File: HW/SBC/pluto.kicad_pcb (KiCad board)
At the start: 2 copper layers, 120.7 x 108 mm, 42 parts, among them J1 Serial Port, J2 CONN_02X07, J3 CONN_02X07, J4 POWER IN, J5 Expansion Port, Q1 DS1813, SW1 RESET, U1 WD65C02_, U10 74LS138, U11 LM7805CT, U2 28C256, U3 HM62256BLP-7, U4 MAX232, U5 6551, U6 WD65C22, U7 DS1511Y+, U8 74HCT00, U9 74LS30, X1 4 MHz

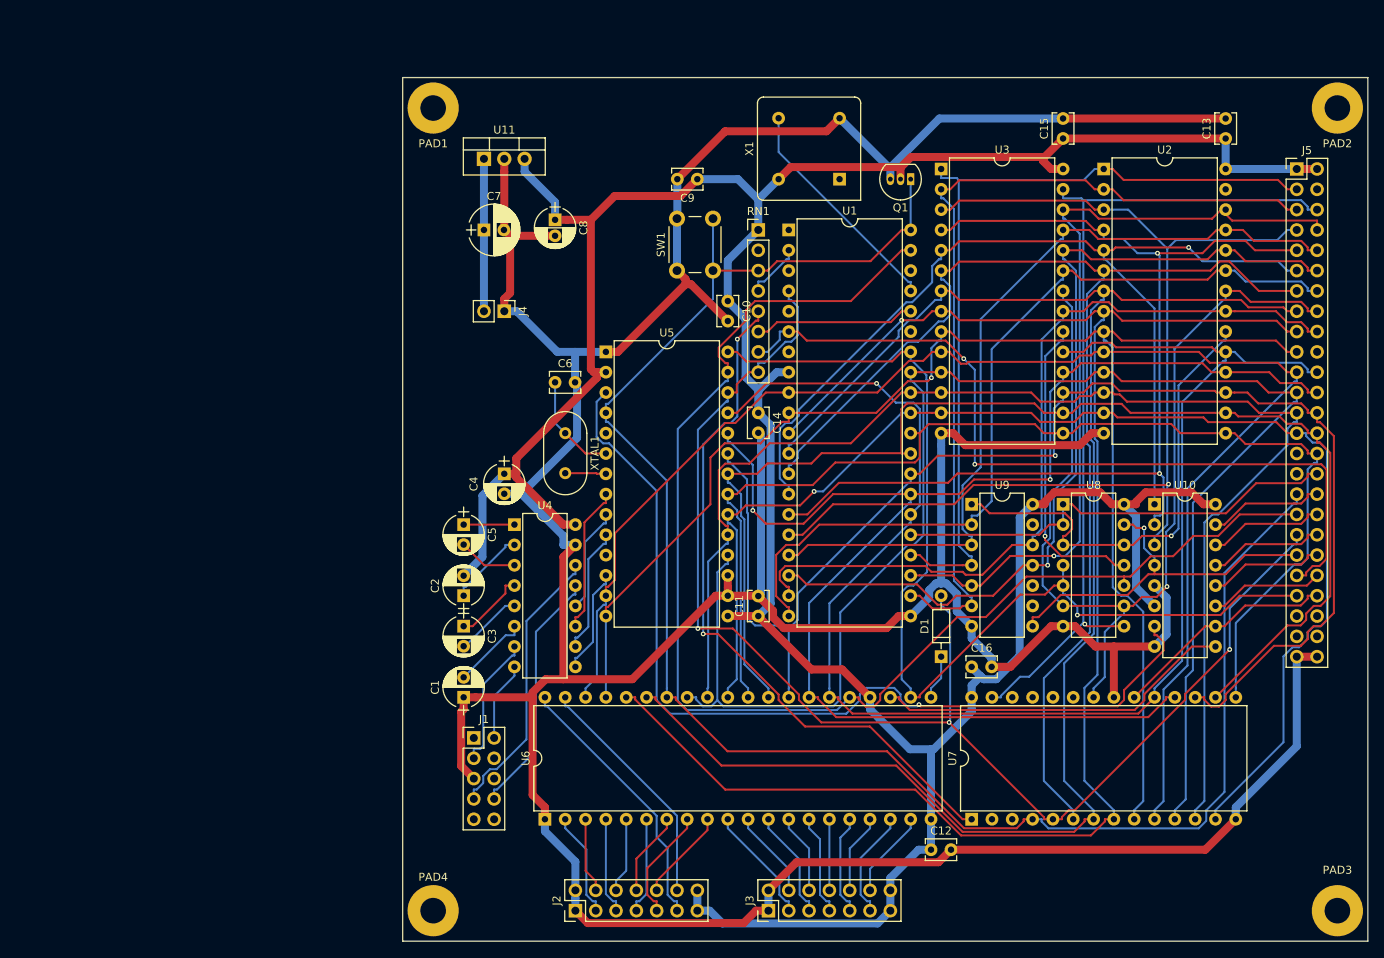
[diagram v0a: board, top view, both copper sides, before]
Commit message: New board layout. WIP
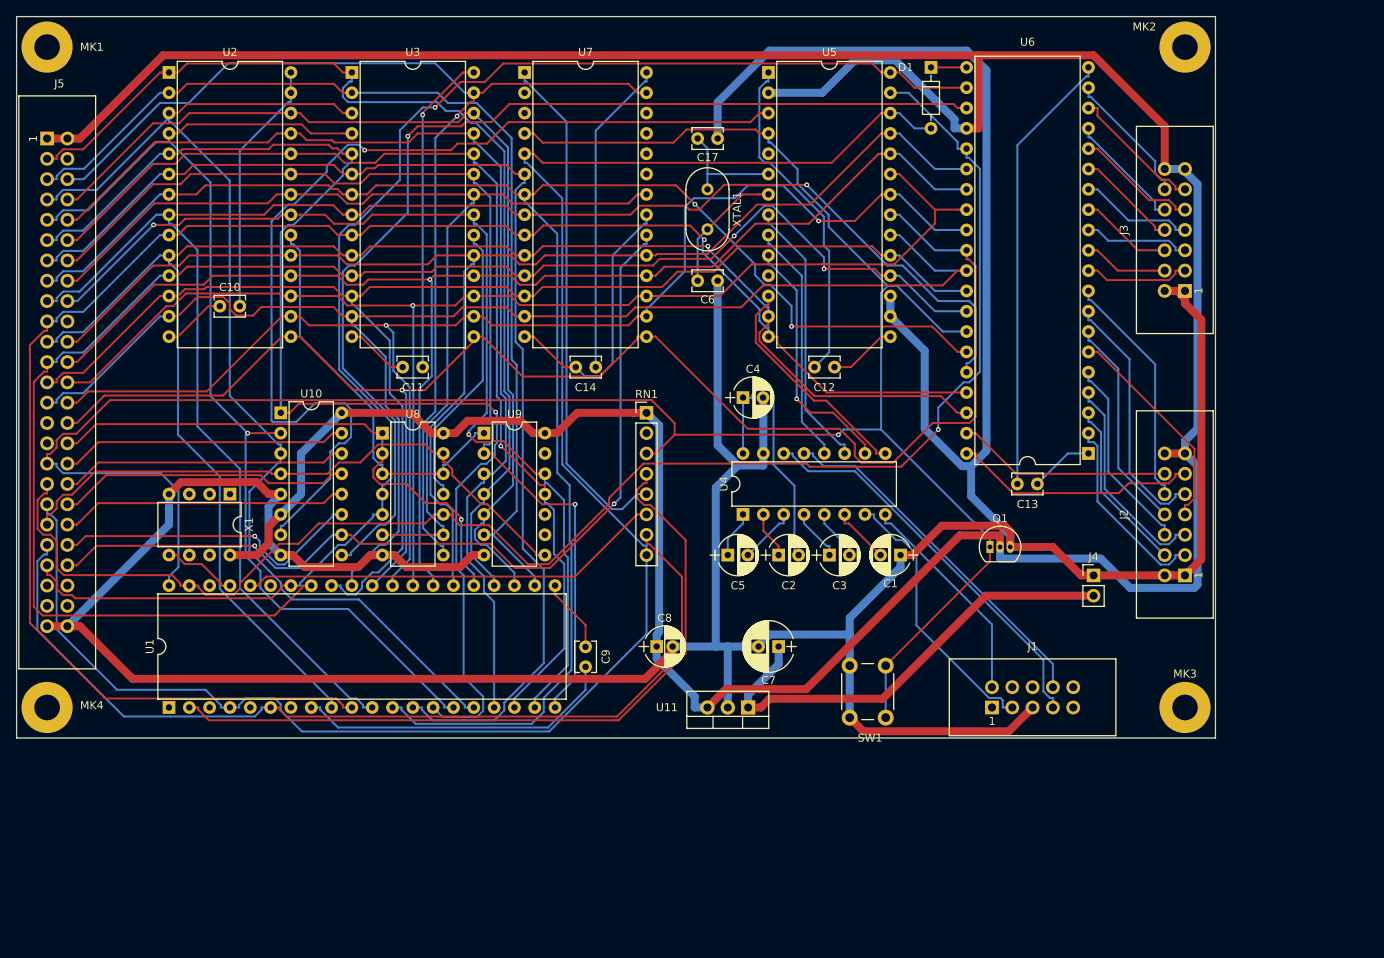
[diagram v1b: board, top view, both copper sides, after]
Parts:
- removed C15, C16: .1uF, Capacitors_ThroughHole:C_Disc_D3.8mm_W2.6mm_P2.50mm
- removed PAD1, PAD2, PAD3, PAD4: MountingHole_3.2mm_M3_Pad, Mounting_Holes:MountingHole_3.2mm_M3_Pad
- added C17: 22pF, Capacitors_ThroughHole:C_Disc_D3.8mm_W2.6mm_P2.50mm, F.Cu at (124.5, 44.5)
- added MK1: Mounting_Hole, Mounting_Holes:MountingHole_3.2mm_M3_Pad, F.Cu at (40.6, 33.0)
- added MK2: Mounting_Hole, Mounting_Holes:MountingHole_3.2mm_M3_Pad, F.Cu at (182.9, 33.0)
- added MK3: Mounting_Hole, Mounting_Holes:MountingHole_3.2mm_M3_Pad, F.Cu at (182.9, 115.6)
- added MK4: Mounting_Hole, Mounting_Holes:MountingHole_3.2mm_M3_Pad, F.Cu at (40.6, 115.6)
- C10, C11, C12, C13, C14, C9: value .1uF -> 0.1uF
- J1: footprint Pin_Headers:Pin_Header_Straight_2x05_Pitch2.54mm -> Connect:IDC_Header_Straight_10pins
- J2, J3: footprint Pin_Headers:Pin_Header_Straight_2x07_Pitch2.54mm -> Connect:IDC_Header_Straight_14pins
- J5: footprint Pin_Headers:Pin_Header_Straight_2x25_Pitch2.54mm -> Connect:IDC_Header_Straight_50pins
- X1: footprint Oscillators:Oscillator_DIP-8 -> Housings_DIP:DIP-8_W7.62mm
- moved J5 156.3 mm to (40.6, 44.5), turned to 270 degrees
- moved U2 117.5 mm to (55.9, 36.2)
- moved U10 109.8 mm to (69.8, 78.7)
- moved U7 108.8 mm to (100.3, 36.2), turned to 0 degrees
- moved U1 97.8 mm to (55.9, 115.6), turned to 90 degrees
- moved J3 93.3 mm to (182.9, 63.5)
- moved J2 87.0 mm to (182.9, 99.1)
- moved X1 85.8 mm to (63.5, 88.9), turned to 270 degrees
- moved U8 85.6 mm to (82.5, 81.3)
- moved U6 81.9 mm to (170.8, 83.8), turned to 180 degrees
- moved J4 80.7 mm to (171.4, 99.1), turned to 0 degrees
- moved U11 76.1 mm to (128.3, 115.6), turned to 180 degrees
- moved U3 74.6 mm to (78.7, 36.2)
- moved D1 73.7 mm to (151.1, 35.6), turned to 270 degrees
- moved J1 64.9 mm to (158.8, 115.6)
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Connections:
- C10 pad 1: VCC -> Net-(C10-Pad1)
- C10 pad 2: GND -> Net-(C10-Pad2)
- C11 pad 1: VCC -> Net-(C11-Pad1)
- C11 pad 2: GND -> Net-(C11-Pad2)
- C12 pad 1: VCC -> Net-(C12-Pad1)
- C12 pad 2: GND -> Net-(C12-Pad2)
- C13 pad 1: VCC -> Net-(C13-Pad1)
- C13 pad 2: GND -> Net-(C13-Pad2)
- C14 pad 1: VCC -> Net-(C14-Pad1)
- C14 pad 2: GND -> Net-(C14-Pad2)
- C2 pad 2: VCC -> Net-(C2-Pad2)
- C4 pad 1: VCC -> Net-(C2-Pad2)
- C6 pad 1: Net-(C6-Pad1) -> GND
- C6 pad 2: GND -> Net-(C6-Pad2)
- C9 pad 1: VCC -> Net-(C9-Pad1)
- C9 pad 2: GND -> Net-(C9-Pad2)
- U1 pad 21: GND -> Net-(C9-Pad2)
- U1 pad 8: VCC -> Net-(C9-Pad1)
- U2 pad 14: GND -> Net-(C10-Pad1)
- U2 pad 27: (no net) -> Net-(C10-Pad2)
- U2 pad 28: VCC -> Net-(C10-Pad2)
- U3 pad 14: GND -> Net-(C11-Pad1)
- U3 pad 28: VCC -> Net-(C11-Pad2)
- U4 pad 16: VCC -> Net-(C2-Pad2)
- U5 pad 1: GND -> Net-(C12-Pad2)
- U5 pad 15: VCC -> Net-(C12-Pad1)
- U5 pad 6: Net-(C6-Pad1) -> Net-(C17-Pad2)
- U5 pad 7: Net-(U5-Pad7) -> Net-(C6-Pad2)
- U6 pad 1: GND -> Net-(C13-Pad2)
- U6 pad 20: VCC -> Net-(C13-Pad1)
- U7 pad 14: GND -> Net-(C14-Pad2)
- U7 pad 21: GND -> Net-(C14-Pad2)
- U7 pad 28: VCC -> Net-(C14-Pad1)
- XTAL1 pad 1: Net-(C6-Pad1) -> Net-(C17-Pad2)
- XTAL1 pad 2: Net-(U5-Pad7) -> Net-(C6-Pad2)
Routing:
- net ~7FCX: track 45.2 -> 134.5 mm, vias 0 -> 1
- net RDY: track 7.26 -> 92.4 mm
- net ~7FAX: track 28.3 -> 112.8 mm, vias 0 -> 2
- net ~RES: track 223.8 -> 281.3 mm, vias 0 -> 1
- net Net-(C13-Pad1): track 0.00 -> 55.9 mm
- net ~IRQ: track 171.0 -> 223.5 mm, vias 3 -> 0
- net D3: track 144.9 -> 197.4 mm, vias 0 -> 1
- net R/~W: track 130.7 -> 180.1 mm
- net Net-(C12-Pad2): track 0.00 -> 42.2 mm
- net Net-(C9-Pad1): track 0.00 -> 40.3 mm
- net Net-(C11-Pad2): track 0.00 -> 40.3 mm, vias 0 -> 1
- net Net-(C14-Pad1): track 0.00 -> 39.6 mm
- net GND: track 544.9 -> 505.8 mm
- net /Power and expansion port/+9V: track 19.1 -> 58.2 mm
- net ~MWR: track 107.2 -> 142.7 mm
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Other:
- board size 120.7 x 108 mm -> 149.9 x 90.2 mm
